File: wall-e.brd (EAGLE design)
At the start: 62.2 x 51.9 mm, 71 parts, among them IC1 VREG-TS1117CW-3V3, T1 BC847, U1 TSM2306CX, U2 TSM2306CX, U3 TSM2306CX, U4 TSM2306CX, U5 TSM2306CX, U6 TSM2306CX, U7 TSM2306CX, U8 LM293AD, U9 TSM2306CX

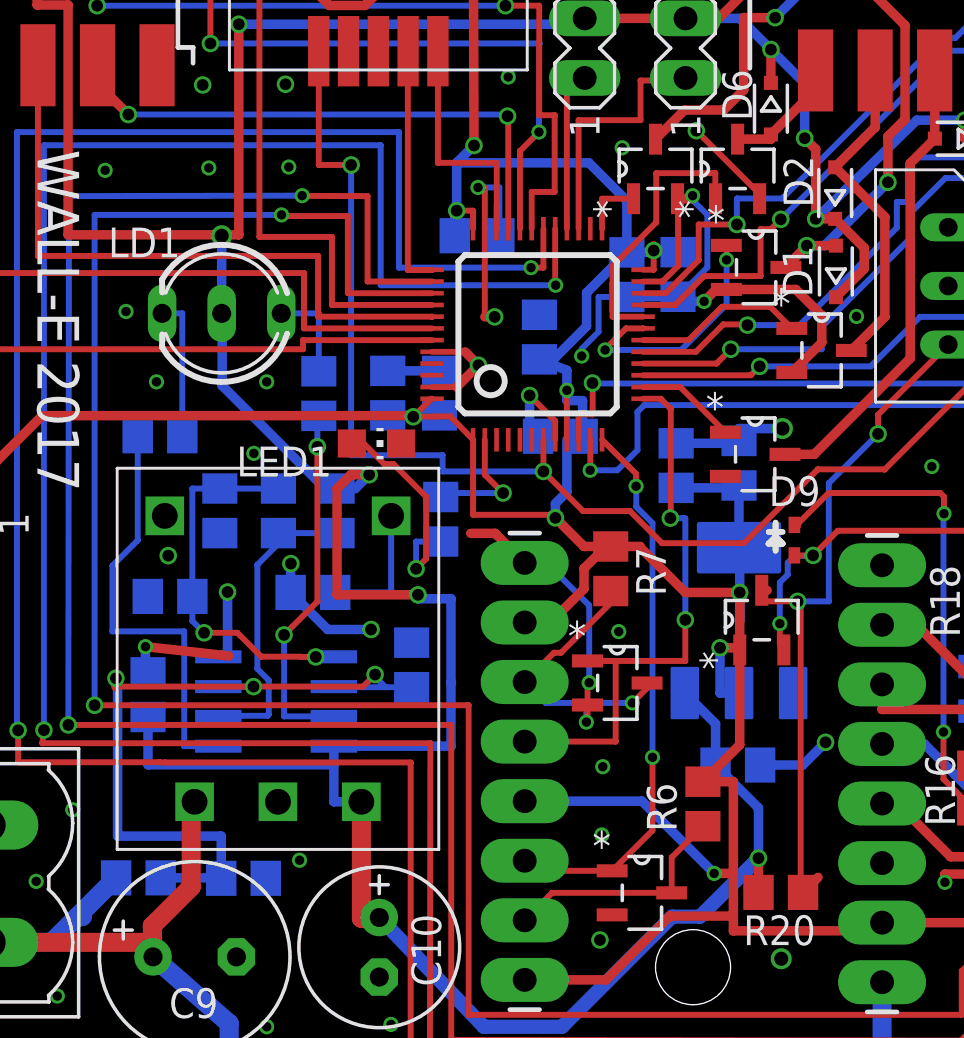
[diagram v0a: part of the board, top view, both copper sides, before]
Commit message: Minor changes
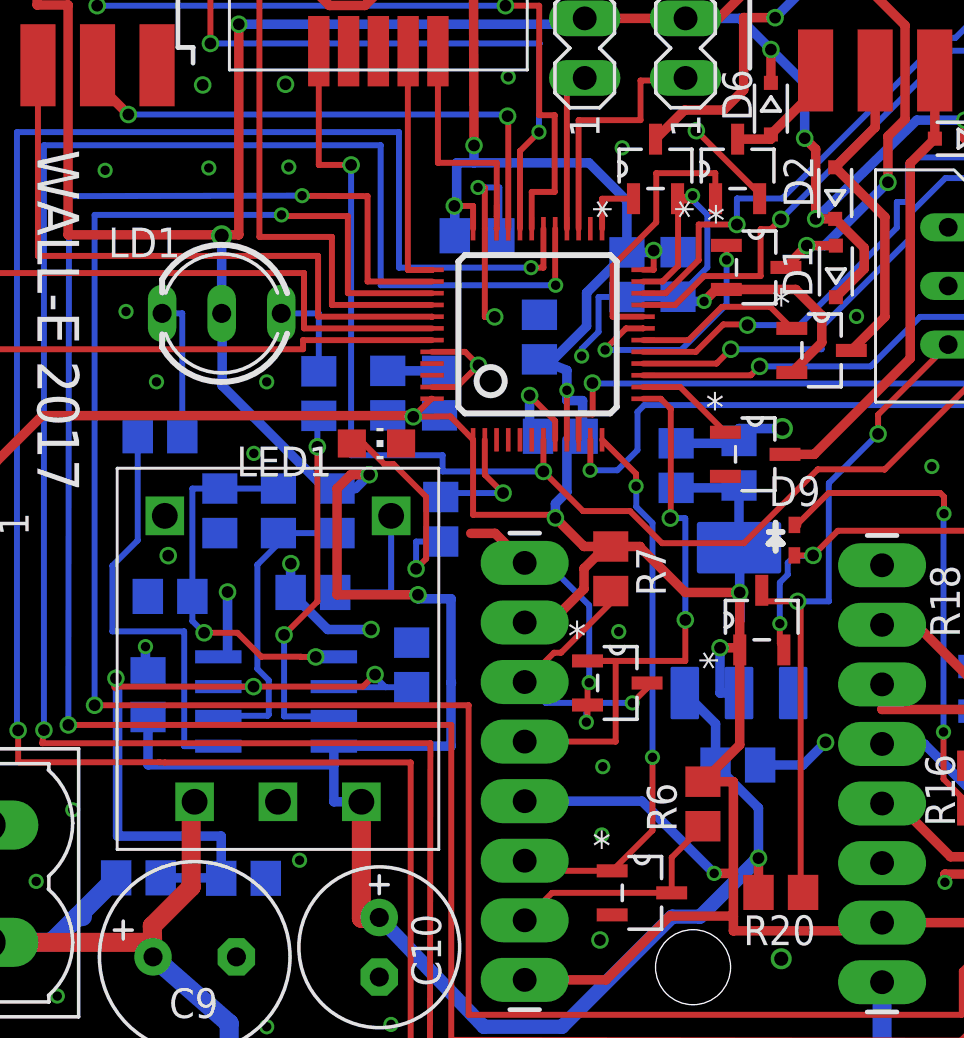
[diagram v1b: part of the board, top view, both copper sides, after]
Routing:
- net GND: track 127.0 -> 123.4 mm
- net N$23: track 47.9 -> 46.8 mm
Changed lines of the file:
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@@
 <wire x1="65.94" y1="35.11" x2="65.83" y2="35.21" width="0.4064" layer="16"/>
 <wire x1="65.83" y1="35.21" x2="65.83" y2="36.21" width="0.4064" layer="16"/>
-<wire x1="65.83" y1="36.21" x2="69.39" y2="35.81" width="0.4064" layer="1"/>
 <via x="75.45" y="36.94" extent="1-16" drill="0.5"/>
 <wire x1="78.05" y1="48.78" x2="79.46" y2="48.78" width="0.254" layer="1"/>
-<wire x1="80.03" y1="48.21" x2="79.46" y2="48.78" width="0.4064" layer="1"/>
+<wire x1="80.03" y1="48.21" x2="79.46" y2="48.78" width="0.254" layer="1"/>
 <via x="80.03" y="48.21" extent="1-16" drill="0.5"/>
 <wire x1="78.05" y1="47.28" x2="79.1" y2="47.28" width="0.254" layer="1"/>
-<wire x1="79.1" y1="47.28" x2="80.03" y2="48.21" width="0.4064" layer="1"/>
+<wire x1="79.1" y1="47.28" x2="80.03" y2="48.21" width="0.254" layer="1"/>
 <wire x1="83.3" y1="45.03" x2="83.3" y2="45.83" width="0.254" layer="1"/>
 <wire x1="83.3" y1="45.83" x2="82.21" y2="46.92" width="0.254" layer="1"/>
@@
 <wire x1="85.15" y1="51.12" x2="86.36" y2="51.12" width="0.254" layer="16"/>
 <wire x1="80.3" y1="54.03" x2="80.3" y2="50.27" width="0.254" layer="1"/>
-<wire x1="80.3" y1="50.27" x2="80.72" y2="50.27" width="0.4064" layer="1"/>
+<wire x1="80.3" y1="50.27" x2="80.72" y2="50.27" width="0.254" layer="1"/>
 <via x="110.22" y="45.38" extent="1-16" drill="0.5"/>
 <wire x1="111.96" y1="48.77" x2="111.96" y2="45.38" width="0.4064" layer="1"/>
@@
 <contactref element="JP2" pad="7"/>
 <contactref element="JP2" pad="4"/>
-<wire x1="87.5" y1="53.1" x2="87.5" y2="53.3" width="0.4064" layer="1"/>
 <via x="87.5" y="53.1" extent="1-16" drill="0.5"/>
 <wire x1="87.5" y1="53.02" x2="86.36" y2="53.02" width="0.4064" layer="16"/>
@@
 <wire x1="87.5" y1="53.1" x2="88.54" y2="53.1" width="0.4064" layer="16"/>
 <wire x1="88.54" y1="53.1" x2="88.54" y2="53.03" width="0.4064" layer="16"/>
-<wire x1="79.8" y1="54.03" x2="79.8" y2="54.8" width="0.254" layer="1"/>
-<wire x1="79.8" y1="54.8" x2="79.1" y2="54.8" width="0.254" layer="1"/>
-<via x="79.1" y="54.8" extent="1-16" drill="0.5"/>
-<wire x1="79.02" y1="54.8" x2="79.1" y2="54.8" width="0.4064" layer="16"/>
+<via x="79" y="55" extent="1-16" drill="0.5"/>
+<wire x1="79.02" y1="54.8" x2="79" y2="55" width="0.4064" layer="16"/>
 <wire x1="79.02" y1="54.8" x2="79.02" y2="53.73" width="0.4064" layer="16"/>
 <wire x1="83.8" y1="45.03" x2="83.8" y2="47.14" width="0.254" layer="1"/>
@@
 <wire x1="79.82" y1="64.08" x2="79.84" y2="57.58" width="0.4064" layer="1"/>
 <via x="79.84" y="57.58" extent="1-16" drill="0.5"/>
-<wire x1="79.1" y1="56.84" x2="79.84" y2="57.58" width="0.4064" layer="16"/>
-<wire x1="79.1" y1="54.8" x2="79.1" y2="56.84" width="0.4064" layer="16"/>
 <wire x1="84.47" y1="45.18" x2="84.86" y2="44.79" width="0.4064" layer="16"/>
 <wire x1="84.86" y1="44.79" x2="84.86" y2="44.64" width="0.4064" layer="16"/>
@@
 <wire x1="84.64" y1="51.3" x2="86.36" y2="53.02" width="0.4064" layer="16"/>
 <wire x1="84.64" y1="49.87" x2="84.64" y2="51.3" width="0.4064" layer="16"/>
-<wire x1="79.1" y1="54.8" x2="79.21" y2="54.8" width="0.4064" layer="16"/>
 <wire x1="86.92" y1="40.48" x2="85.67" y2="40.48" width="0.4064" layer="1"/>
 <wire x1="86.92" y1="40.48" x2="86.92" y2="40.45" width="0.4064" layer="1"/>
@@
 <wire x1="101.37" y1="24.44" x2="97.24" y2="24.44" width="0.4064" layer="1"/>
 <wire x1="86.36" y1="53.02" x2="86.36" y2="55.22" width="0.4064" layer="16"/>
-<wire x1="84.74" y1="56.84" x2="79.1" y2="56.84" width="0.4064" layer="16"/>
+<wire x1="84.74" y1="56.84" x2="79.84" y2="56.84" width="0.4064" layer="16"/>
 <wire x1="86.36" y1="55.22" x2="84.74" y2="56.84" width="0.4064" layer="16"/>
 <wire x1="84.47" y1="46.7" x2="83.8" y2="46.7" width="0.4064" layer="16"/>
@@
 <wire x1="90.08" y1="26.54" x2="90.88" y2="26.54" width="0.4064" layer="1"/>
 <wire x1="90.88" y1="26.54" x2="90.9" y2="26.52" width="0.4064" layer="1"/>
+<wire x1="79" y1="55" x2="79.8" y2="55" width="0.254" layer="1"/>
+<wire x1="79.8" y1="55" x2="79.8" y2="54.03" width="0.254" layer="1"/>
+<wire x1="79" y1="55" x2="79.1" y2="55" width="0.4064" layer="16"/>
+<wire x1="79.1" y1="55" x2="79.1" y2="56.84" width="0.4064" layer="16"/>
+<wire x1="79.1" y1="56.84" x2="79.84" y2="56.84" width="0.4064" layer="16"/>
+<wire x1="79.84" y1="56.84" x2="79.84" y2="57.58" width="0.4064" layer="16"/>
 </signal>
 <signal name="VALVE1">
@@
 <via x="97.07" y="45.28" extent="1-16" drill="0.5"/>
 <via x="93.64" y="38.14" extent="1-16" drill="0.5"/>
-<wire x1="94.51" y1="26.37" x2="93.87" y2="25.73" width="0.4064" layer="1"/>
 <wire x1="100.06" y1="49.09" x2="100.33" y2="49.36" width="0.254" layer="16"/>
 <wire x1="100.33" y1="49.36" x2="105.29" y2="49.36" width="0.254" layer="16"/>
@@
 <wire x1="111.22" y1="44.58" x2="111.22" y2="42.76" width="0.254" layer="1"/>
 <wire x1="111.22" y1="42.76" x2="111.23" y2="42.76" width="0.4064" layer="1"/>
-<wire x1="92.34" y1="38.61" x2="92.11" y2="38.61" width="0.4064" layer="1"/>
 <wire x1="93.87" y1="25.73" x2="93.77" y2="25.83" width="0.254" layer="1"/>
 <wire x1="93.77" y1="38.01" x2="93.77" y2="25.83" width="0.254" layer="1"/>
